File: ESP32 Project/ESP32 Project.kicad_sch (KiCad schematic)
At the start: 12 parts, among them P1 USB_C_Plug_USB2.0, U1 ESP32-S3-WROOM-1-N8R2, U2 AMS1117, U3 BMP390, U4 INA219AxD, U5 LM75B, U6 SHTC3

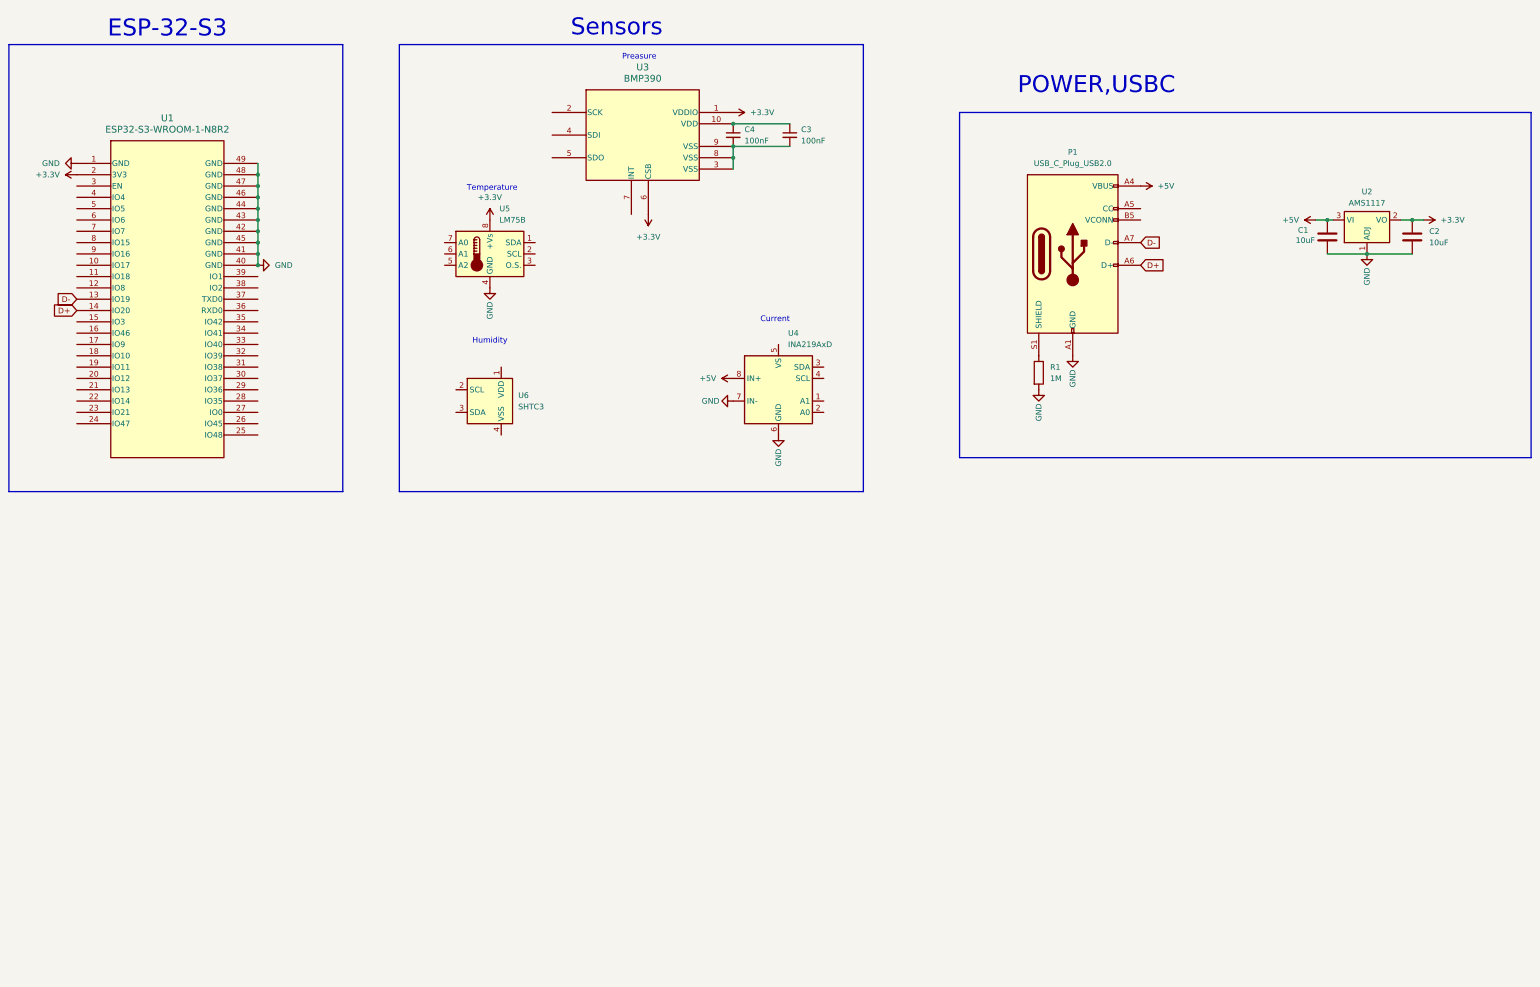
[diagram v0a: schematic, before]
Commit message: added alot, pcb first prototype 4 layers
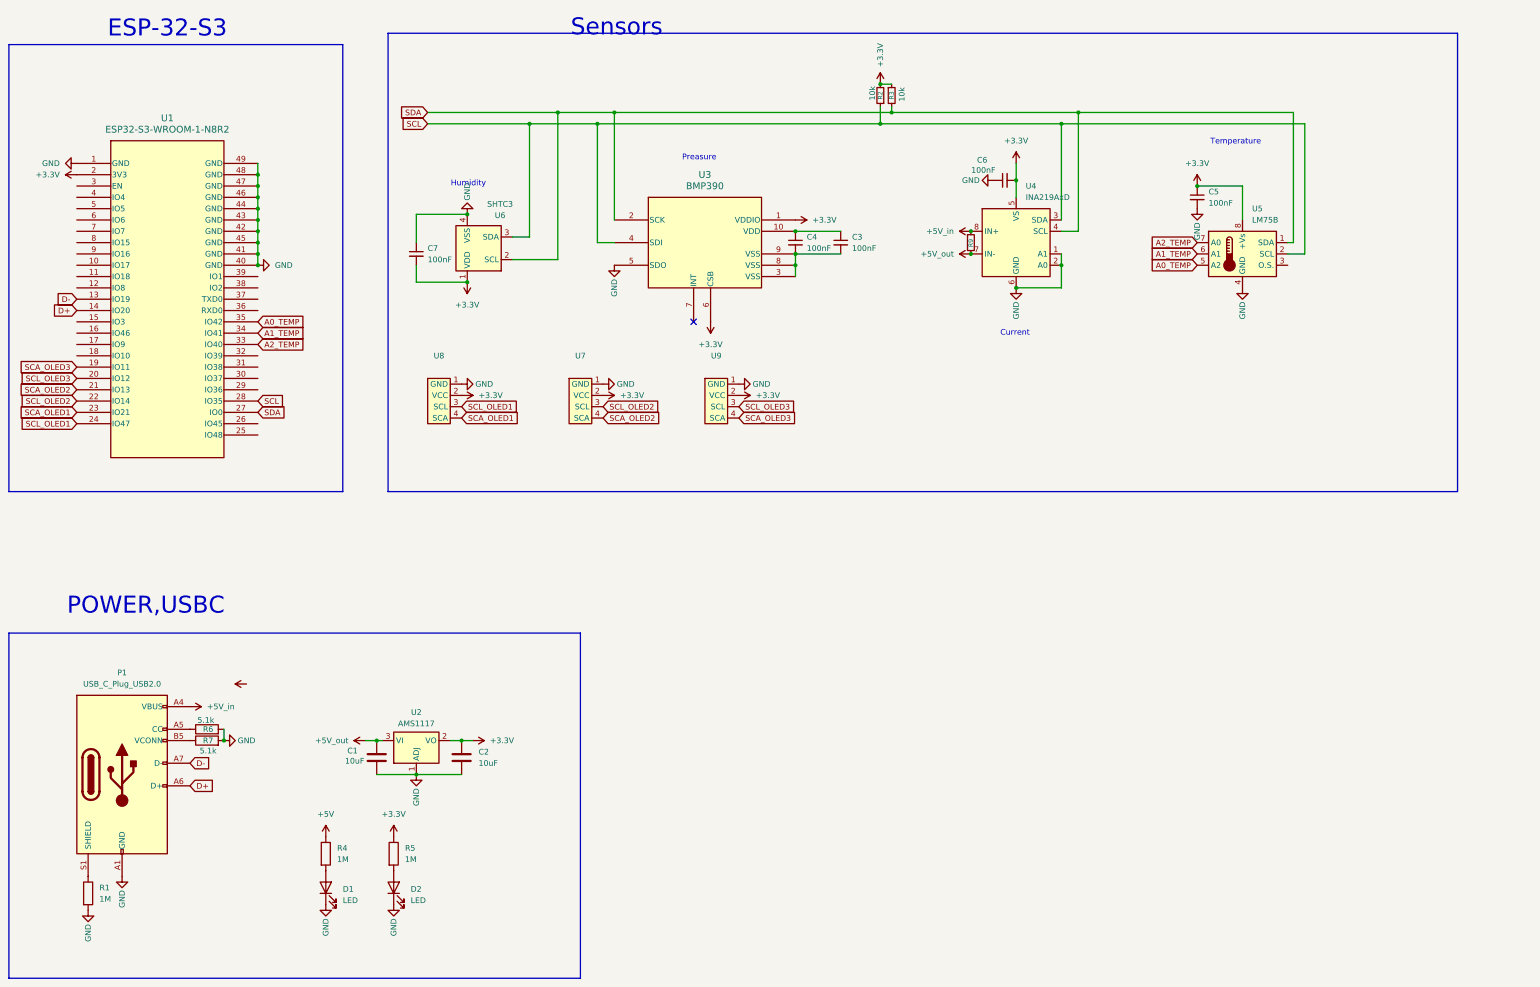
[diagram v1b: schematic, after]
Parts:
- added C5, C6, C7: 100nF, Capacitor_SMD:C_0805_2012Metric_Pad1.18x1.45mm_HandSolder, symbol Device:C_Small
- added D1, D2: LED, LED_SMD:LED_0805_2012Metric_Pad1.15x1.40mm_HandSolder, symbol Device:LED
- added R2, R3: 10k, LED_SMD:LED_0805_2012Metric_Pad1.15x1.40mm_HandSolder, symbol Device:R_Small
- added R4, R5: 1M, Resistor_SMD:R_0805_2012Metric_Pad1.20x1.40mm_HandSolder, symbol Device:R
- added R6, R7: 5.1k, Resistor_SMD:R_0805_2012Metric_Pad1.20x1.40mm_HandSolder, symbol Device:R
- added R9: R_Small, Resistor_SMD:R_0805_2012Metric_Pad1.20x1.40mm_HandSolder, symbol Device:R_Small
- added U7, U8, U9: ~, Connector_PinHeader_2.54mm:PinHeader_1x04_P2.54mm_Vertical, symbol 2025-10-05_20-13-18:pinheader3x
- P1: footprint (none) -> 0custom:USB4105-GF-A-120
- U3: footprint 10LGA_2X2X0p75_BOS -> 0custom:BMP390
- U5: footprint (none) -> 0custom:LM75BD,118
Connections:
- net +3.3V: now also U4.5 (VS), U6.1 (VDD), C5.1, C6.2, C7.2, R2.2, R3.1, R5.1, U7.2 (VCC), U8.2 (VCC), U9.2 (VCC)
- net +5V: now also R4.1; no longer C1.1, P1.A4 (VBUS), P1.A9 (VBUS), P1.B4 (VBUS), P1.B9 (VBUS), U2.3 (VI), U4.8 (IN+)
- net GND: now also U3.5 (SDO), U4.1 (A1), U4.2 (A0), U6.4 (VSS), C5.2, C6.1, C7.1, D1.1 (K), D2.1 (K), R6.2, R7.2, U7.1 (GND), U8.1 (GND), U9.1 (GND); no longer U4.7 (IN-)
- net SDA: now reaches U6.2 (SCL)
- net SDA: now also U1.27 (IO0), U3.2 (SCK), U4.4 (SCL), U5.1 (SDA), R3.2
- net SCL: now reaches U6.3 (SDA)
- net SCL: now also U1.28 (IO35), U3.4 (SDI), U4.3 (SDA), U5.2 (SCL), R2.1
- net at P1.A5 (CC): now also R6.1
- net at P1.B5 (VCONN): now also R7.1
- net SCA_OLED3: now reaches U1.19 (IO11)
- net SCA_OLED3: now also U9.4 (SCA)
- net SCL_OLED3: now reaches U1.20 (IO12)
- net SCL_OLED3: now also U9.3 (SCL)
- net SCA_OLED2: now reaches U1.21 (IO13)
- net SCA_OLED2: now also U7.4 (SCA)
- net SCL_OLED2: now reaches U1.22 (IO14)
- net SCL_OLED2: now also U7.3 (SCL)
- net SCA_OLED1: now reaches U1.23 (IO21)
- net SCA_OLED1: now also U8.4 (SCA)
- net SCL_OLED1: now reaches U1.24 (IO47)
- net SCL_OLED1: now also U8.3 (SCL)
- net A2_TEMP: now reaches U1.33 (IO40)
- net A2_TEMP: now also U5.7 (A0)
- net A1_TEMP: now reaches U1.34 (IO41)
- net A1_TEMP: now also U5.6 (A1)
- net A0_TEMP: now reaches U1.35 (IO42)
- net A0_TEMP: now also U5.5 (A2)
- new net: D1.2 (A), R4.2
- new net: D2.2 (A), R5.2
- new net +5V_in: P1.A4 (VBUS), P1.A9 (VBUS), P1.B4 (VBUS), P1.B9 (VBUS), R9.1, U4.8 (IN+)
- new net +5V_out: C1.1, R9.2, U2.3 (VI), U4.7 (IN-)
- no-connect marks 0 -> 1
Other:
- moved on the sheet: C1, C2, C3, C4, P1, R1, U2, U3, U4, U5, U6

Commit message: newstuff
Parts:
- removed U7, U9: ~, Connector_PinHeader_2.54mm:PinHeader_1x04_P2.54mm_Vertical, symbol 2025-10-05_20-13-18:pinheader3x
- added C8: 100nF, Capacitor_SMD:C_0805_2012Metric_Pad1.18x1.45mm_HandSolder, symbol Device:C_Small
- added JP1, JP10, JP11, JP12, JP13, JP14, JP15, JP16, JP17, JP18, JP19, JP2, JP20, JP21, JP3, JP4, JP5, JP6, JP7, JP8, JP9: SolderJumper_2_Open, Jumper:SolderJumper-2_P1.3mm_Open_RoundedPad1.0x1.5mm, symbol Jumper:SolderJumper_2_Open
- added U7: CCS811, Package_LGA:AMS_LGA-10-1EP_2.7x4mm_P0.6mm, symbol Sensor_Gas:CCS811
- U8: footprint Connector_PinHeader_2.54mm:PinHeader_1x04_P2.54mm_Vertical -> Connector_PinHeader_2.54mm:PinHeader_1x14_P2.54mm_Vertical
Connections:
- net +3.3V: now also U8.1 (VCC), U8.8 (LED), C8.2, JP19.1 (A), JP20.1 (A), JP21.1 (A), U7.6 (VDD); no longer U8.2 (VCC)
- net A0_TEMP: no longer U5.5 (A2)
- net A1_TEMP: no longer U5.6 (A1)
- net A2_TEMP: no longer U5.7 (A0)
- net GND: now also U8.2 (GND), C8.1, JP16.1 (A), JP17.1 (A), JP18.1 (A), U7.1 (ADDR), U7.11 (GND), U7.7 (~{WAKE}); no longer U8.1 (GND)
- net SCL: now also U1.17 (IO9), U7.10 (SCL); no longer U1.28 (IO35)
- net SDA: now also U1.12 (IO8), U7.9 (SDA); no longer U1.27 (IO0)
- net at U1.10 (IO17): now also U8.11 (T_CS)
- net at U1.11 (IO18): now also U8.14 (T_IRQ)
- net at U1.18 (IO10): now also JP9.1 (A)
- net at U1.4 (IO4): now also U8.3 (CS)
- net at U1.5 (IO5): now also U8.4 (RESET)
- net at U1.6 (IO6): now also U8.5 (DC/RS)
- net at U1.7 (IO7): now also U8.12 (T_DIN), U8.6 (SDI(MOSI))
- net at U1.8 (IO15): now also U8.10 (T_CLK), U8.7 (SCK)
- net at U1.9 (IO16): now also U8.13 (T_DO), U8.9 (SDO(MISO))
- net at U3.7 (INT): now also JP1.1 (A)
- net at U5.3 (O.S.): now also JP5.1 (A)
- net SCA_OLED1: no longer names the net of U1.23 (IO21)
- net SCA_OLED1: now also JP14.1 (A); no longer U8.4 (SCA)
- net SCA_OLED2: no longer names the net of U1.21 (IO13)
- net SCA_OLED2: now also JP12.1 (A)
- net SCA_OLED3: no longer names the net of U1.19 (IO11)
- net SCA_OLED3: now also JP10.1 (A)
- net SCL_OLED1: no longer names the net of U1.24 (IO47)
- net SCL_OLED1: now also JP15.1 (A); no longer U8.3 (SCL)
- net SCL_OLED2: no longer names the net of U1.22 (IO14)
- net SCL_OLED2: now also JP13.1 (A)
- net SCL_OLED3: no longer names the net of U1.20 (IO12)
- net SCL_OLED3: now also JP11.1 (A)
- new net: JP6.1 (A), U7.2 (~{RESET})
- new net: JP7.1 (A), U7.3 (~{INT})
- new net: U7.4 (PWM), U7.5 (Sense)
- new net: JP8.1 (A), U7.8 (AUX)
- new net: JP3.1 (A), U5.6 (A1)
- new net: JP2.1 (A), U5.7 (A0)
- new net: JP4.1 (A), U5.5 (A2)
- no-connect marks 1 -> 20
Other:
- moved on the sheet: C1, C2, C3, C4, C5, C6, C7, D1, D2, P1, R1, R2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
